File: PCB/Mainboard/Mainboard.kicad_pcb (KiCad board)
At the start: 2 copper layers, 1 part, among them J1 Conn_GPS

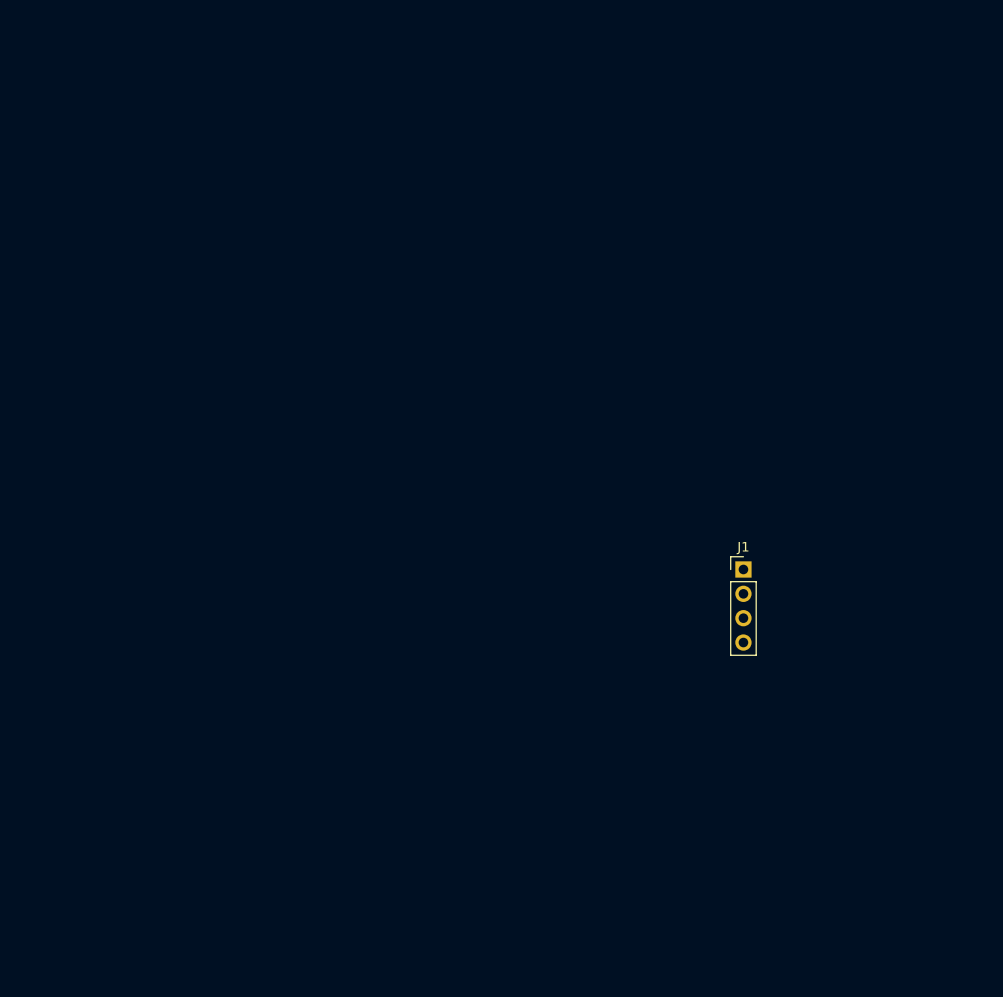
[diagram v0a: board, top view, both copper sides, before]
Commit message: First rev is done
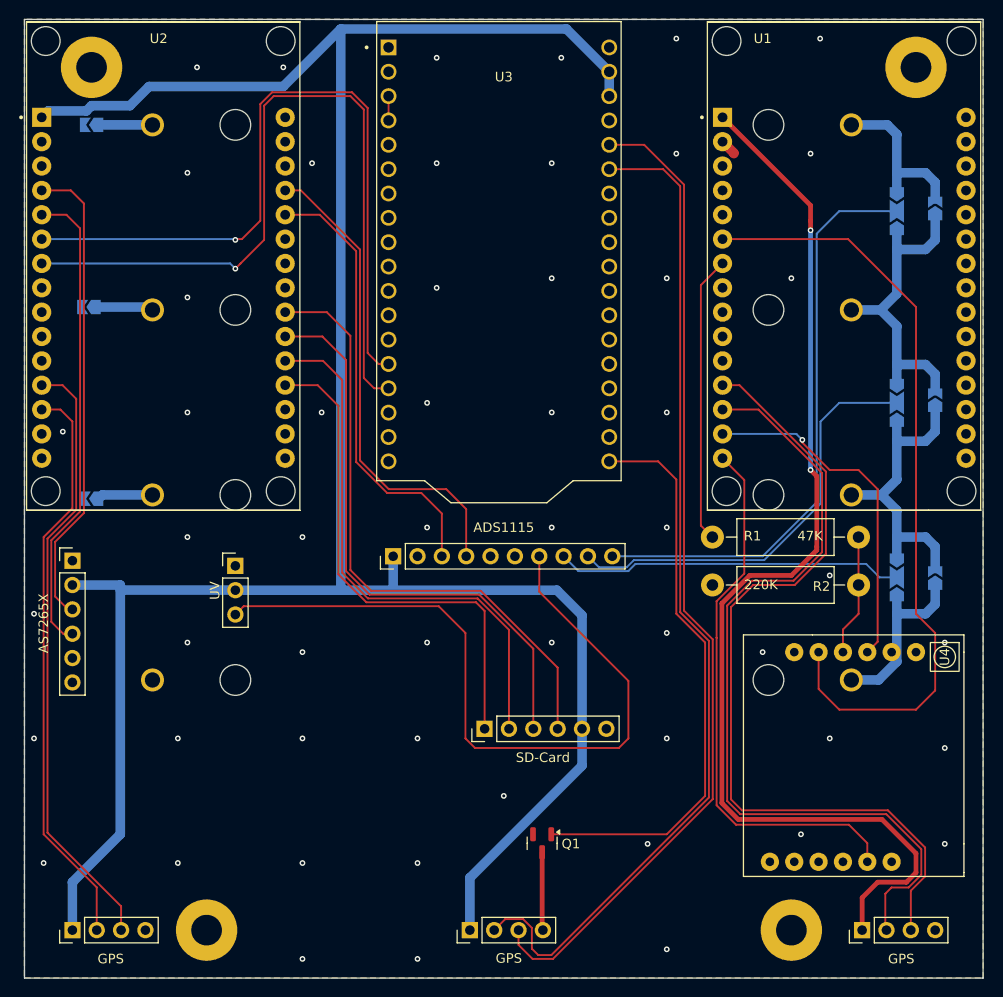
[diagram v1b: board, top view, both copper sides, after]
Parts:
- added BT1: BK-18650-PC8, Felix:BAT_BK-18650-PC8, B.Cu at (112.8, 67.0)
- added H1: MountingHole_Pad, MountingHole:MountingHole_3.2mm_M3_Pad, F.Cu at (70.0, 32.0)
- added H2: MountingHole_Pad, MountingHole:MountingHole_3.2mm_M3_Pad, F.Cu at (156.0, 32.0)
- added H3: MountingHole_Pad, MountingHole:MountingHole_3.2mm_M3_Pad, F.Cu at (143.0, 122.0)
- added H4: MountingHole_Pad, MountingHole:MountingHole_3.2mm_M3_Pad, F.Cu at (82.0, 122.0)
- added J2: AS7265X, Connector_PinHeader_2.54mm:PinHeader_1x06_P2.54mm_Vertical, F.Cu at (68.0, 83.5)
- added J3: UV, Connector_PinHeader_2.54mm:PinHeader_1x03_P2.54mm_Vertical, F.Cu at (85.0, 84.0)
- added J4: ADS1115, Connector_PinHeader_2.54mm:PinHeader_1x10_P2.54mm_Vertical, F.Cu at (101.5, 83.0)
- added J5: GPS, Connector_PinHeader_2.54mm:PinHeader_1x04_P2.54mm_Vertical, F.Cu at (68.0, 122.0)
- added J6: GPS, Connector_PinHeader_2.54mm:PinHeader_1x04_P2.54mm_Vertical, F.Cu at (109.5, 122.0)
- added J7: SD-Card, Connector_PinHeader_2.54mm:PinHeader_1x06_P2.54mm_Vertical, F.Cu at (111.0, 101.0)
- added JP1: SolderJumper_3_Open, Jumper:SolderJumper-3_P2.0mm_Open_TrianglePad1.0x1.5mm_NumberLabels, B.Cu at (154.0, 67.0)
- added JP10: SolderJumper_2_Open, Jumper:SolderJumper-2_P1.3mm_Open_TrianglePad1.0x1.5mm, B.Cu at (158.0, 66.7)
- added JP11: SolderJumper_2_Open, Jumper:SolderJumper-2_P1.3mm_Open_TrianglePad1.0x1.5mm, B.Cu at (158.0, 85.3)
- added JP2: SolderJumper_3_Open, Jumper:SolderJumper-3_P2.0mm_Open_TrianglePad1.0x1.5mm_NumberLabels, B.Cu at (154.0, 47.0)
- added JP3: SolderJumper_3_Open, Jumper:SolderJumper-3_P2.0mm_Open_TrianglePad1.0x1.5mm_NumberLabels, B.Cu at (154.0, 85.2)
- added JP4: SolderJumper_2_Open, Jumper:SolderJumper-2_P1.3mm_Open_TrianglePad1.0x1.5mm, B.Cu at (70.0, 38.0)
- added JP5: SolderJumper_2_Open, Jumper:SolderJumper-2_P1.3mm_Open_TrianglePad1.0x1.5mm, B.Cu at (69.7, 57.0)
- added JP6: SolderJumper_2_Open, Jumper:SolderJumper-2_P1.3mm_Open_TrianglePad1.0x1.5mm, B.Cu at (70.0, 77.0)
- added JP9: SolderJumper_2_Open, Jumper:SolderJumper-2_P1.3mm_Open_TrianglePad1.0x1.5mm, B.Cu at (158.0, 46.7)
- added Q1: AO3400A, Package_TO_SOT_SMD:SOT-23, F.Cu at (117.0, 112.9)
- added R1: 47K, Resistor_THT:R_Axial_DIN0411_L9.9mm_D3.6mm_P15.24mm_Horizontal, F.Cu at (134.8, 81.0)
- added R2: 220K, Resistor_THT:R_Axial_DIN0411_L9.9mm_D3.6mm_P15.24mm_Horizontal, F.Cu at (150.0, 86.0)
- added U1: ESP32-DEVKIT-V1, Felix:MODULE_ESP32_DEVKIT_V1_NO_WIFI, F.Cu at (148.5, 52.7)
- added U2: ESP32-DEVKIT-V1, Felix:MODULE_ESP32_DEVKIT_V1_NO_WIFI, F.Cu at (77.5, 52.7)
- added U3: WIFI_KIT_32__V3_, Felix:MODULE_WIFI_KIT_32__V3_, F.Cu at (112.5, 52.3)
- added U4: SIM800L-CORE, Felix_GSM:SIM800L-CORE, F.Cu at (156.0, 93.0)
- J1: value Conn_GPS -> GPS
- moved J1 39.6 mm to (150.4, 122.0), turned to 90 degrees
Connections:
- J1 pad 1: +3.3V -> /GPSModule/VCC
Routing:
- net +3.3V: track 0.00 -> 259.5 mm
- net /GPSModule/VCC: track 0.00 -> 116.8 mm, vias 0 -> 2
- net /RX: track 0.00 -> 105.7 mm
- net /TX: track 0.00 -> 104.2 mm
- net /GPSModule/RX: track 0.00 -> 87.4 mm
- net /GPSModule/TX: track 0.00 -> 86.9 mm
- net /GsmModule/TX: track 0.00 -> 81.7 mm
- net Net-(U2-TX2): track 0.00 -> 81.1 mm, vias 0 -> 1
- net /ADS1115/A0: track 0.00 -> 77.2 mm
- net Net-(U2-RX2): track 0.00 -> 76.4 mm, vias 0 -> 1
- net /SdCard/MISO: track 0.00 -> 64.5 mm
- net /GPSModule1/TX: track 0.00 -> 64.0 mm
- net /ADS1115/A3: track 0.00 -> 61.0 mm
- net /SdCard/MOSI: track 0.00 -> 60.6 mm
- net /GPSModule1/RX: track 0.00 -> 60.3 mm
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- added copper zone on B.Cu, net GND
- added copper zone on F.Cu, net GND
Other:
- board outline added: 100 x 100 mm
- board text added: "+"
- board text added: "-"
- board text added: "Diese Batterie spreist GSM"
